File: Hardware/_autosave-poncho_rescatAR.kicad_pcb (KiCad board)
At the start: 2 copper layers, 10 parts, among them P2 CONN_8, Q1 BC547

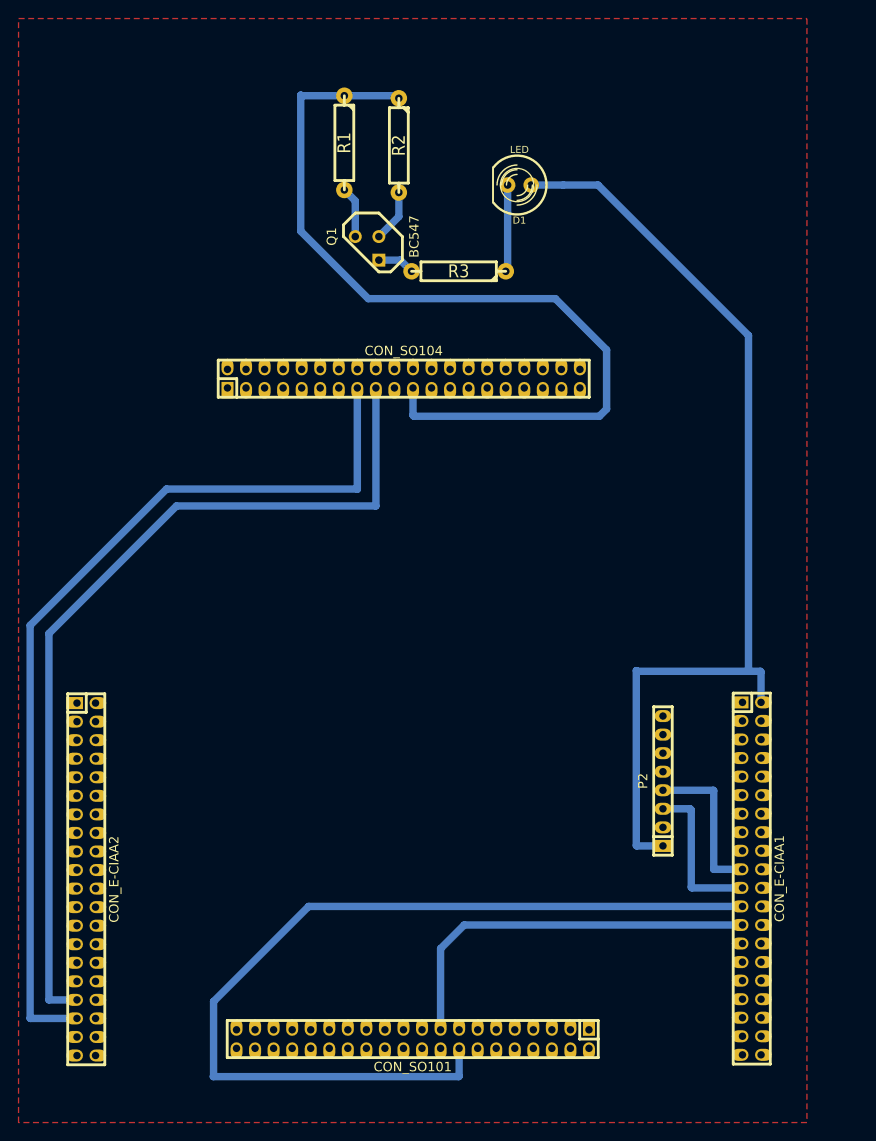
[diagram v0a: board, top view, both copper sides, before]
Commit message: retoques finales al esquemetico y pcb base
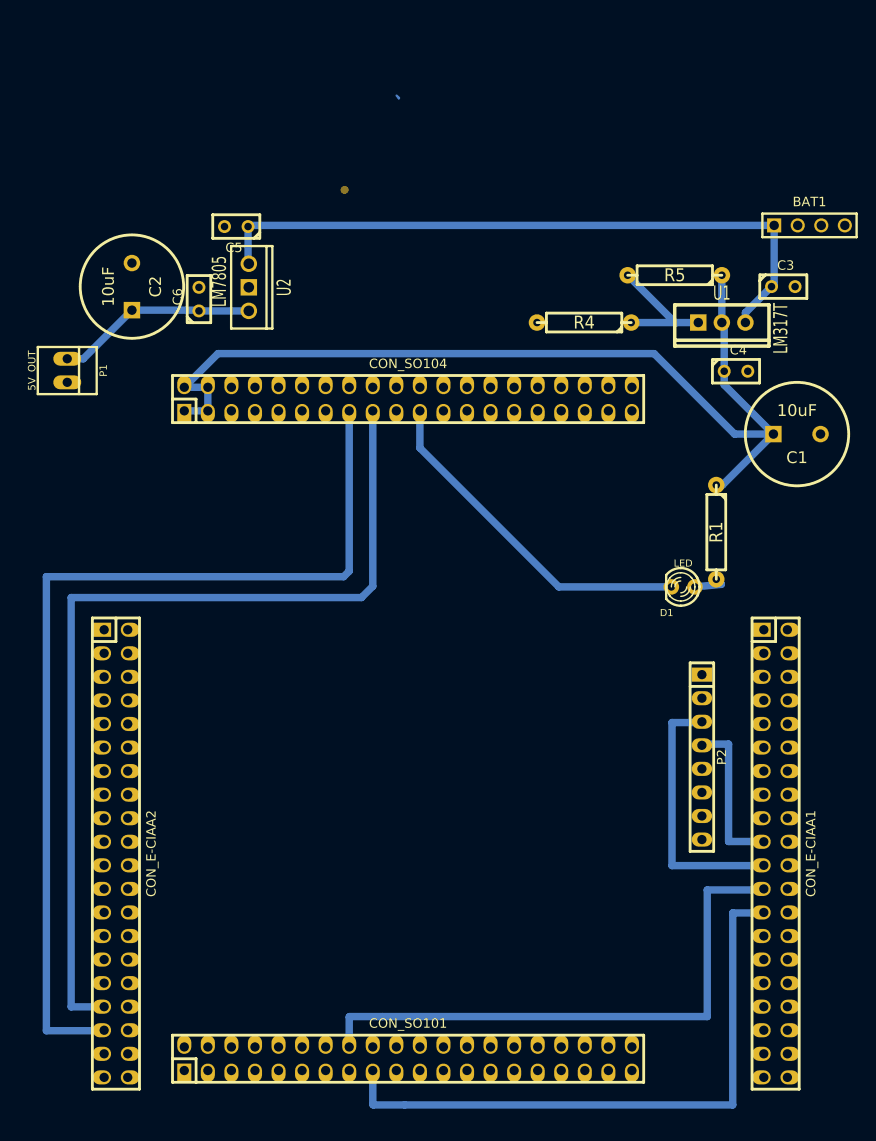
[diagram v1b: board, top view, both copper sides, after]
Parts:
- removed Q1: BC547, TO92
- removed R2: 10k, R4-LARGE_PADS
- removed R3: 680, R4-LARGE_PADS
- added BAT1: BAT_CONN, PIN_ARRAY_4x1, F.Cu at (165.3, 52.3)
- added C1: 10uF, C2V10, F.Cu at (163.9, 74.8)
- added C2: 10uF, C2V10, F.Cu at (92.2, 58.9)
- added C3: 0.1, C1, F.Cu at (162.4, 58.9)
- added C4: 0.1, C1, F.Cu at (157.3, 68.0)
- added C5: 0.1, C1, F.Cu at (103.5, 52.4)
- added C6: 0.1, C1, F.Cu at (99.5, 60.2)
- added P1: 5V_OUT, PINHEAD1-2, F.Cu at (85.2, 67.9)
- added R4: 470, R4-LARGE_PADS, F.Cu at (141.0, 62.8)
- added R5: 220, R4-LARGE_PADS, F.Cu at (150.8, 57.6)
- added U1: LM317T, TO220_VERT, F.Cu at (155.8, 62.8)
- added U2: LM7805, LM78XXV, F.Cu at (104.8, 59.0)
- CON_E-CIAA1, CON_E-CIAA2, CON_SO101, CON_SO104: footprint pin_strip_2mm_20x2 -> pin_strip_20x2
- D1: footprint LED-5MM -> LED-3MM
- P2: footprint pin_socket_2mm_8 -> pin_strip_8
- R1: value 330k -> 330
- moved R1 58.1 mm to (155.2, 85.3)
- moved D1 46.8 mm to (151.7, 91.2)
- moved P2 4.93 mm to (153.7, 109.6), turned to 270 degrees
- moved CON_E-CIAA2 4.24 mm to (90.5, 120.0)
- moved CON_E-CIAA1 3.73 mm to (161.6, 120.0)
- moved CON_SO104 2.25 mm to (122.0, 71.0)
- moved CON_SO101 2.18 mm to (122.0, 142.1), turned to 0 degrees
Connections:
- CON_E-CIAA1 pad 20: GND -> /GND
- CON_E-CIAA1 pad 22: GND -> /GND
- CON_E-CIAA1 pad 24: GND -> /GND
- CON_E-CIAA1 pad 26: GND -> /GND
- CON_E-CIAA1 pad 28: GND -> /GND
- CON_E-CIAA1 pad 30: GND -> /GND
- CON_E-CIAA1 pad 32: GND -> /GND
- CON_E-CIAA1 pad 38: GND -> /GND
- CON_E-CIAA1 pad 4: GND -> /GND
- CON_E-CIAA1 pad 40: GND -> /GND
- CON_E-CIAA2 pad 11: GND -> /GND
- CON_E-CIAA2 pad 13: GND -> /GND
- CON_E-CIAA2 pad 17: GND -> /GND
- CON_E-CIAA2 pad 19: GND -> /GND
- CON_E-CIAA2 pad 25: GND -> /GND
- CON_E-CIAA2 pad 27: GND -> /GND
- CON_E-CIAA2 pad 3: GND -> /GND
- CON_E-CIAA2 pad 37: GND -> /GND
- CON_E-CIAA2 pad 39: GND -> /GND
- CON_E-CIAA2 pad 5: GND -> /GND
- CON_E-CIAA2 pad 7: GND -> /GND
- CON_SO101 pad 11: GND -> /GND
- CON_SO101 pad 12: GND -> /GND
- CON_SO101 pad 13: GND -> /GND
- CON_SO101 pad 14: GND -> /GND
- CON_SO101 pad 19: GND -> /GND
- CON_SO101 pad 25: GND -> /GND
- CON_SO101 pad 26: GND -> /GND
- CON_SO101 pad 27: GND -> /GND
- CON_SO101 pad 28: GND -> /GND
- CON_SO101 pad 38: GND -> /GND
- CON_SO101 pad 39: GND -> /GND
- CON_SO101 pad 40: GND -> /GND
- CON_SO101 pad 5: GND -> /GND
- CON_SO104 pad 11: GND -> /GND
- CON_SO104 pad 12: GND -> /GND
- CON_SO104 pad 13: GND -> /GND
- CON_SO104 pad 14: GND -> /GND
- CON_SO104 pad 25: GND -> /GND
- CON_SO104 pad 26: GND -> /GND
- CON_SO104 pad 27: GND -> /GND
- CON_SO104 pad 28: GND -> /GND
- CON_SO104 pad 38: GND -> /GND
- CON_SO104 pad 39: GND -> /GND
- CON_SO104 pad 40: GND -> /GND
- CON_SO104 pad 5: GND -> /GND
- CON_SO104 pad 6: GND -> /GND
- CON_SO104 pad 7: GND -> /GND
- CON_SO104 pad 8: GND -> /GND
- D1 pad 1: /VCC_5V -> N-0000018
- D1 pad 2: N-000005 -> /STATUS_LED
- P2 pad 2: GND -> /GND
- P2 pad 7: GND -> /GND
- R1 pad 1: /STATUS_LED -> /VCC_3.8V
- R1 pad 2: GND -> N-0000018
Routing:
- net /VCC_5V: track 104.9 -> 0.00 mm
- net /VCC_3.8V: track 0.00 -> 104.1 mm
- net VCC: track 0.00 -> 72.6 mm
- net /STATUS_LED: track 94.7 -> 37.3 mm
- net /RS232_RXD: track 98.9 -> 61.6 mm
- net /RS232_TXD: track 42.4 -> 66.6 mm
- net N-000003: track 0.00 -> 21.8 mm
- net N-000002: track 0.00 -> 14.6 mm
- net /I2C_SCL: track 17.0 -> 28.6 mm
- net N-000005: track 9.38 -> 0.00 mm
- net GND: track 6.08 -> 0.00 mm
- net N-000007: track 5.64 -> 0.00 mm
- net /GE864_ON_OFF: track 99.8 -> 105.4 mm
- net N-000009: track 4.02 -> 0.00 mm
- net N-0000018: track 0.00 -> 3.63 mm
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- removed copper zone on F.Cu, net GND
